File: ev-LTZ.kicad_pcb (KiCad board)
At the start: 2 copper layers, 50 x 100 mm, 35 parts, among them P1 VIN+, P2 CONN_01X02, P3 VH-, P4 VH+, P5 SENSE-, P6 SENSE+, P7 VIN-, Q1 BD139, U1 LT1013N8

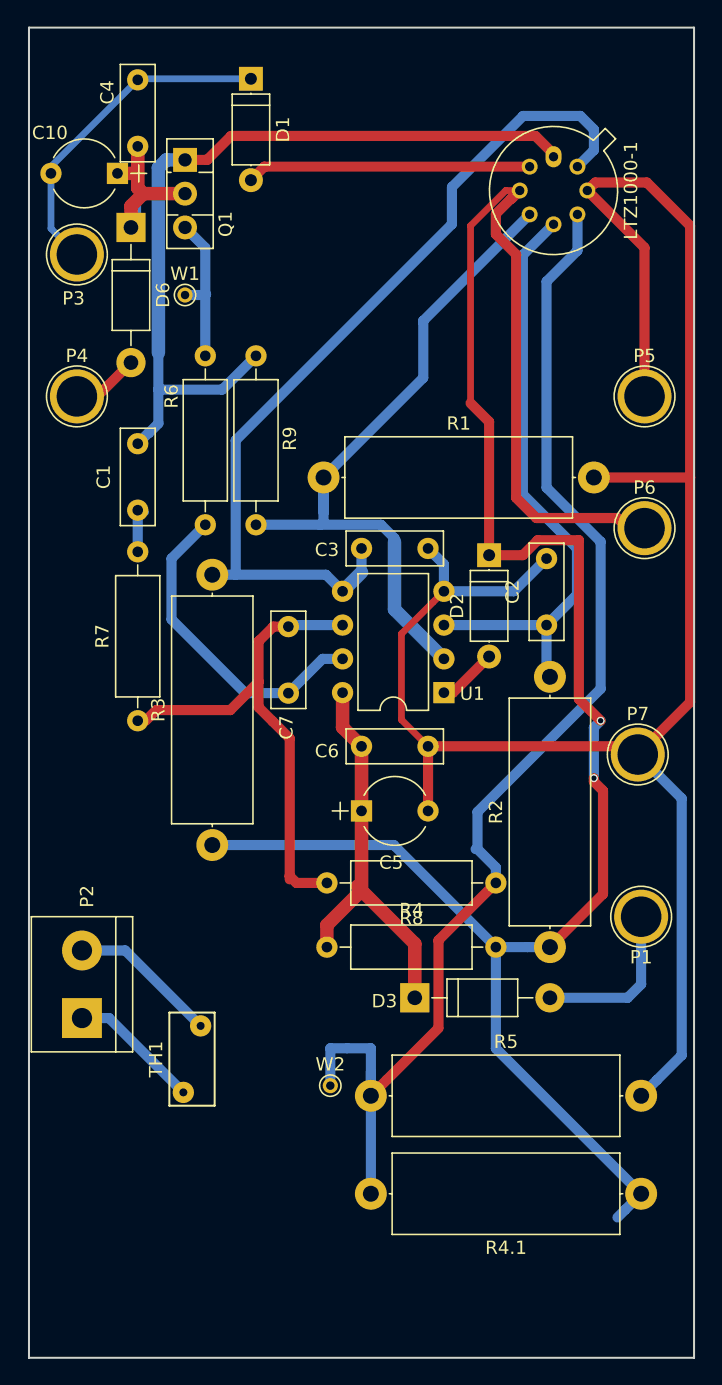
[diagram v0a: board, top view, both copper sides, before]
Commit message: improve traces
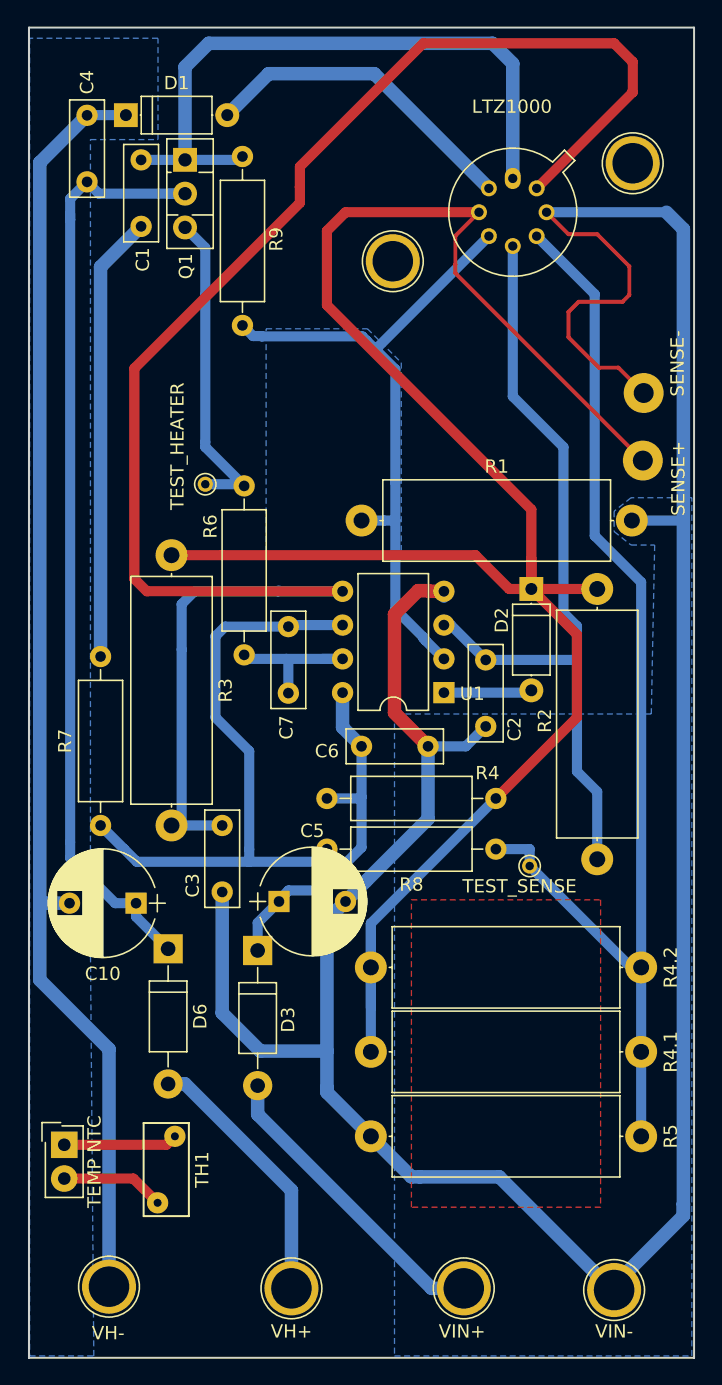
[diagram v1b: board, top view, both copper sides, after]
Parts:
- added R4.2: 25k, Resistors_THT:R_Axial_DIN0617_L17.0mm_D6.0mm_P20.32mm_Horizontal, F.Cu at (155.7, 120.7)
- added REF**: 1pin, Connectors:1pin, F.Cu at (157.4, 67.6)
- added REF**: 1pin, Connectors:1pin, F.Cu at (175.4, 60.2)
- C10, C5: footprint Capacitors_THT:CP_Radial_Tantal_D5.0mm_P5.00mm -> Capacitors_THT:CP_Radial_D8.0mm_P5.00mm
- P2: value CONN_01X02 -> TEMP NTC; footprint Connectors:bornier2 -> Connectors_Samtec:SL-102-X-XX_1x02
- P5, P6: footprint Connectors:1pin -> Measurement_Points:Measurement_Point_Round-TH_Big
- R4.1: value 12k -> 25k
- moved P3 77.6 mm to (136.0, 144.7)
- moved P4 69.0 mm to (149.7, 144.8)
- moved C10 54.9 mm to (138.0, 115.8)
- moved D6 54.3 mm to (140.5, 119.3)
- moved P7 40.3 mm to (174.0, 144.9)
- moved P1 31.0 mm to (162.7, 144.8)
- moved R2 27.2 mm to (172.7, 92.2), turned to 270 degrees
- moved C3 23.3 mm to (144.5, 110.0), turned to 270 degrees
- moved R4.1 23.0 mm to (155.7, 127.0), turned to 0 degrees
- moved W2 22.3 mm to (167.6, 113.0)
- moved R3 22.0 mm to (140.7, 89.7), turned to 270 degrees
- moved C1 21.3 mm to (138.4, 64.9)
- moved R5 20.5 mm to (176.0, 133.3), turned to 180 degrees
- moved R9 15.0 mm to (146.1, 72.4)
- moved W1 14.3 mm to (143.3, 84.3)
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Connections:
- net /VCC renamed /VCCH
- net Net-(C5-Pad1) renamed /VCCOPAMP
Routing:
- net GND: track 151.2 -> 233.0 mm
- net /VH-: track 25.2 -> 96.9 mm
- net /TSENSE_C: track 66.6 -> 127.2 mm
- net /VCCH: track 19.1 -> 72.0 mm
- net Net-(C1-Pad1): track 3.08 -> 33.6 mm
- net /VH+: track 5.12 -> 20.0 mm
- net /TCOMP: track 45.4 -> 59.8 mm
- net Net-(C7-Pad2): track 24.4 -> 12.1 mm
- net /HEAT: track 11.9 -> 24.0 mm
- net /HEATER+: track 61.6 -> 49.6 mm
- net /VIN+: track 12.4 -> 23.1 mm
- net /TSENSE_B: track 95.9 -> 86.3 mm
- net Net-(C7-Pad1): track 38.4 -> 46.5 mm
- net /SENSE+: track 160.7 -> 154.2 mm, vias 2 -> 0
- net /ZENER-: track 55.8 -> 50.8 mm
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- added copper zone on F.Cu, net (none)
- added copper zone on B.Cu, net /VH-
- added copper zone on B.Cu, net /ZENER-
- added copper zone on B.Cu, net GND
- removed copper zone on B.Cu, net /TSENSE
